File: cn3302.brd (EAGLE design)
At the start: 44 x 23 mm, 20 parts, among them M1 CN3302SOP-8

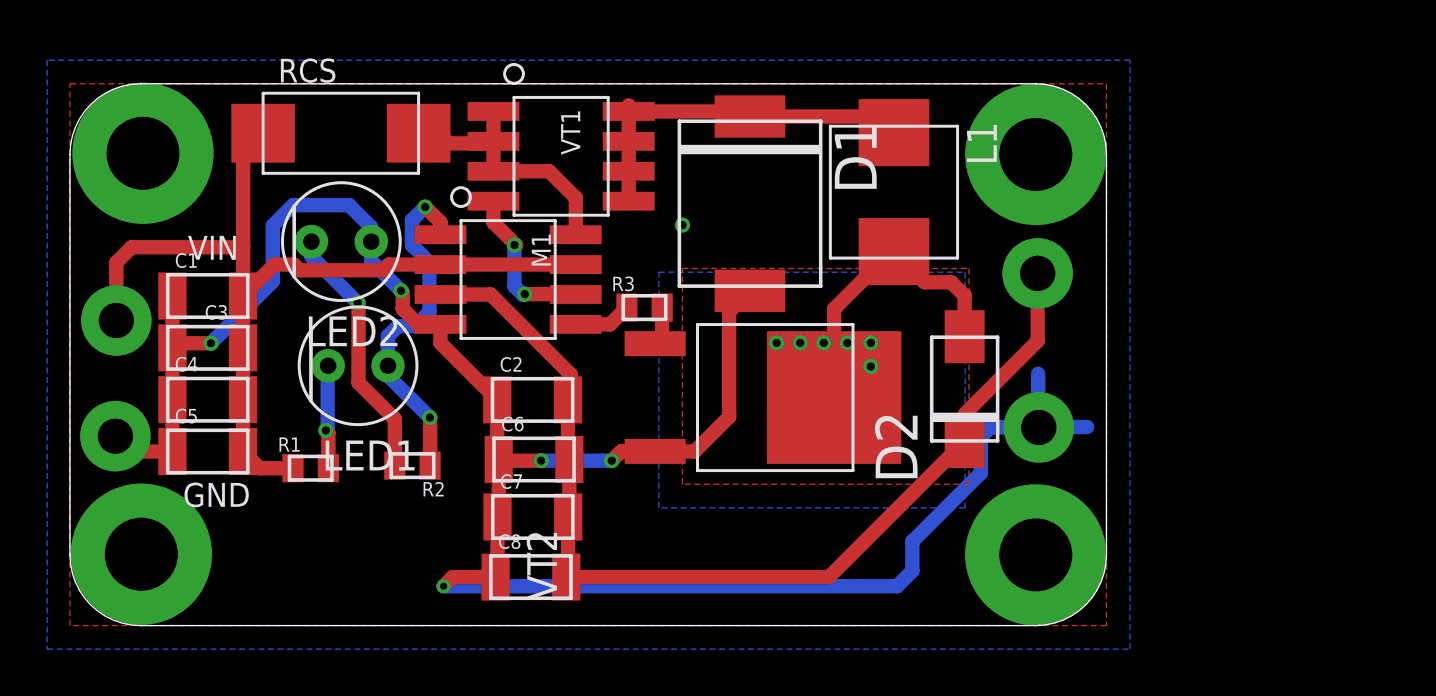
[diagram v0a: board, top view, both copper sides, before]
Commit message: исправил плату
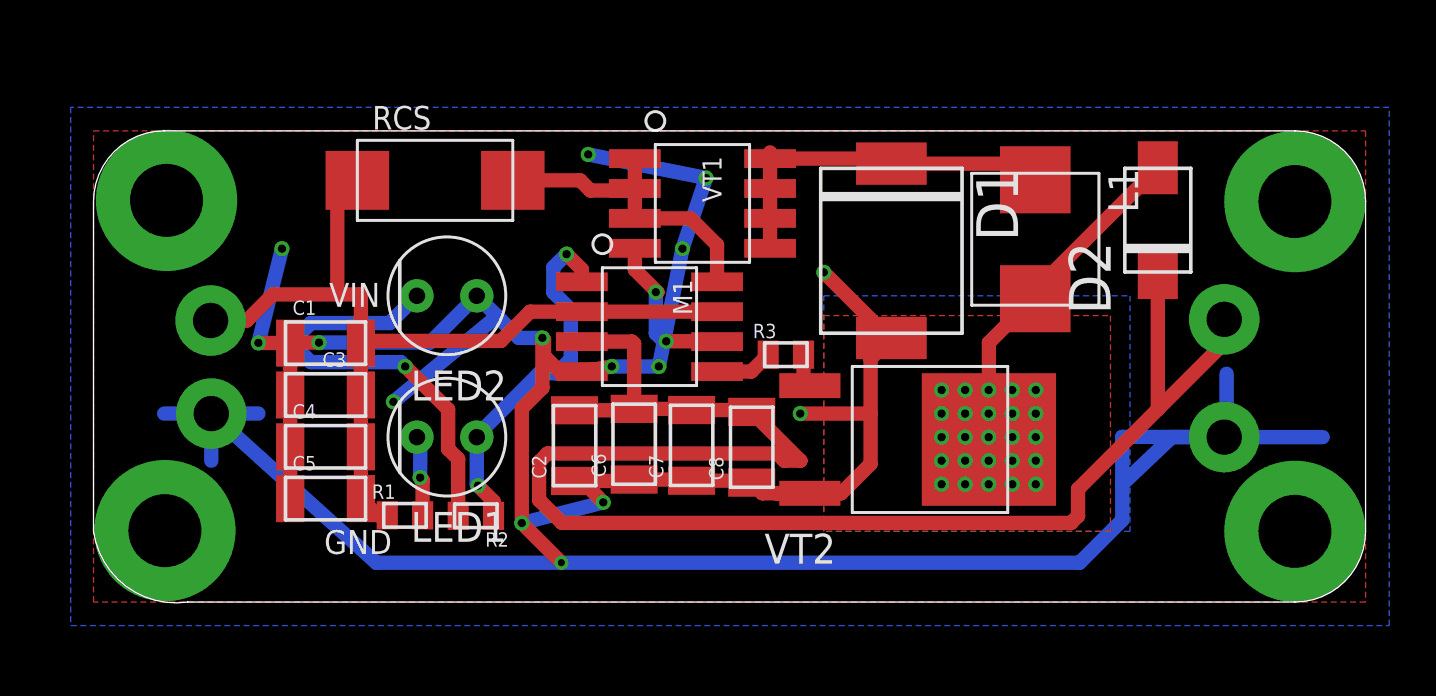
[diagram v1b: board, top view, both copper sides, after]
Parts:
- moved D2 10.9 mm to (45.2, 17.2)
- moved C8 10.9 mm to (27.9, 7.57), turned to 90 degrees
- moved C7 7.39 mm to (25.4, 7.65), turned to 90 degrees
- moved VT2 6.81 mm to (35.5, 7.90)
- moved L1 6.32 mm to (40.0, 16.4)
- moved M1 6.32 mm to (23.6, 12.7)
- moved R3 6.32 mm to (29.4, 11.5)
- moved VT1 6.32 mm to (25.9, 17.9)
- moved D1 6.32 mm to (33.9, 15.9)
- moved C1 5.39 mm to (9.85, 12.0)
- moved C3 5.39 mm to (9.85, 9.79)
- moved C4 5.39 mm to (9.85, 7.59)
- moved C5 5.39 mm to (9.85, 5.39)
- moved LED2 5.04 mm to (15.0, 14.0)
- moved LED1 4.84 mm to (15.0, 8.00)
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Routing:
- net GND: track 96.4 -> 161.7 mm, vias 7 -> 15
- net 8.4V: track 42.3 -> 68.9 mm
- net N$2: track 11.0 -> 18.4 mm
- net N$6: track 11.5 -> 13.5 mm
- net 5V: track 39.6 -> 37.8 mm
- net N$10: track 12.9 -> 14.6 mm, vias 6 -> 25
- net N$1: track 4.43 -> 3.42 mm
- net N$5: track 15.0 -> 15.6 mm
- added copper zone on layer 16, net N$10
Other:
- board size 44 x 23 mm -> 54 x 20 mm
